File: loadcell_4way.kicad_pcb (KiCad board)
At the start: 2 copper layers, 60 x 40 mm, 76 parts, among them J1 USB_B_Micro, J2 Battery, J3 OLDED_Screen, J4 Load Cell, Q1 FDS6892A, Q2 BSS138, Q3 SM2331PSA P-MOSFET, Q4 S8550, Q5 BSS138, SW1 SW_Push, SW2 SW_Push, SW3 SW_Push, U1 FS312F-G, U2 MT3608, U3 TP4056, U4 CH330N, U5 LM1117-3.3, U7 HX711

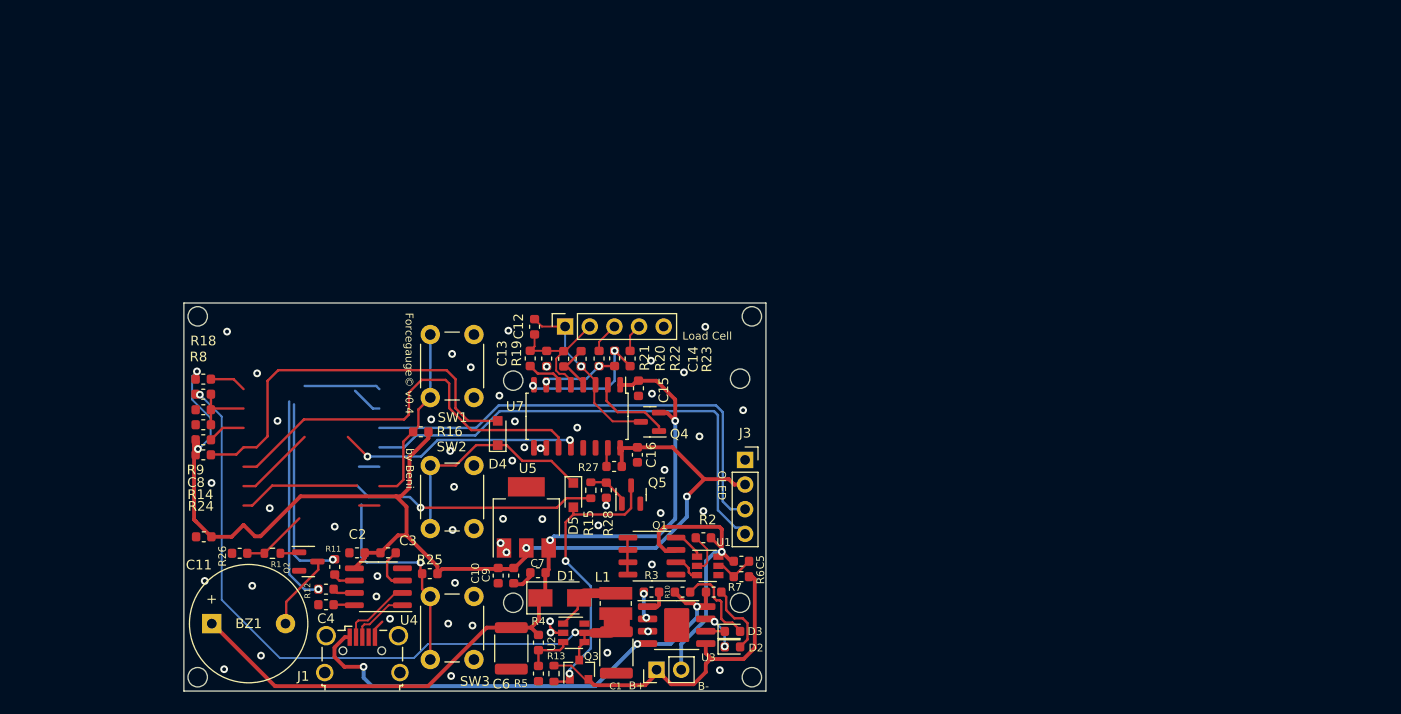
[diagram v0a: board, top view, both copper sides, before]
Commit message: wip
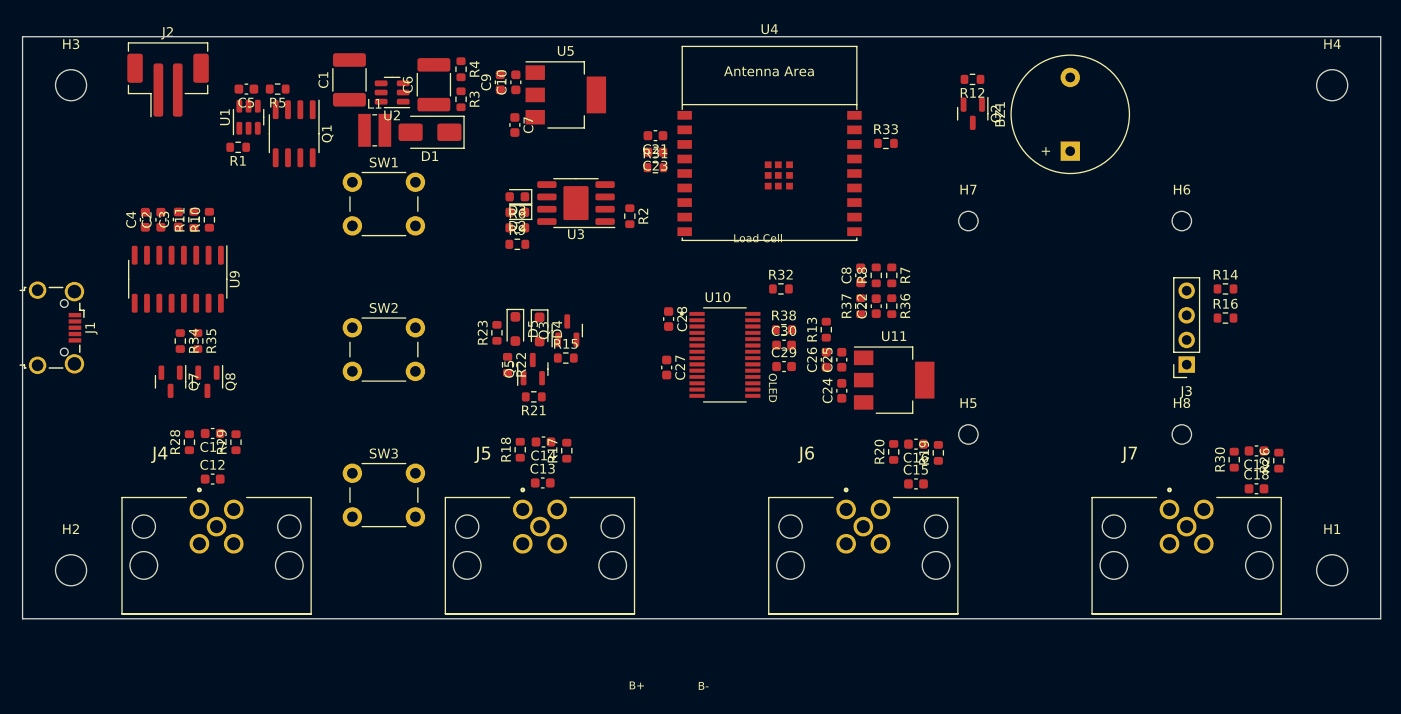
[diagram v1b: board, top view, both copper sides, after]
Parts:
- removed C11: 100nF, Capacitor_SMD:C_0603_1608Metric
- removed Q4: S8550, Package_TO_SOT_SMD:SOT-23
- removed R24: 100k, Resistor_SMD:R_0603_1608Metric
- removed R25: 10k, Resistor_SMD:R_0603_1608Metric
- removed R27: 0R, Resistor_SMD:R_0603_1608Metric
- removed U7: HX711, Package_SO:SOP-16_4.55x10.3mm_P1.27mm
- added C17: 100nF, Capacitor_SMD:C_0603_1608Metric, F.Cu at (119.6, 80.9)
- added C18: 100nF, Capacitor_SMD:C_0603_1608Metric, F.Cu at (227.2, 86.6)
- added C19: 100nF, Capacitor_SMD:C_0603_1608Metric, F.Cu at (227.2, 82.7)
- added C21: 100nF, Capacitor_SMD:C_0603_1608Metric, F.Cu at (165.2, 50.2)
- added C22: 100nF, Capacitor_SMD:C_0603_1608Metric, F.Cu at (188.0, 67.8)
- added C23: 10uF, Capacitor_SMD:C_0603_1608Metric, F.Cu at (165.2, 51.9)
- added C24: 10uF, Capacitor_SMD:C_0603_1608Metric, F.Cu at (184.4, 76.5)
- added C25: 10uF, Capacitor_SMD:C_0603_1608Metric, F.Cu at (184.4, 73.3)
- added C26: 100nF, Capacitor_SMD:C_0603_1608Metric, F.Cu at (182.8, 73.3)
- added C27: 100nF, Capacitor_SMD:C_0603_1608Metric, F.Cu at (166.4, 74.1)
- added C28: 100nF, Capacitor_SMD:C_0603_1608Metric, F.Cu at (166.6, 69.1)
- added C29: 100nF, Capacitor_SMD:C_0603_1608Metric, F.Cu at (178.5, 74.0)
- added C30: 100nF, Capacitor_SMD:C_0603_1608Metric, F.Cu at (178.5, 71.8)
- added J5: T4145015051-001, Loadcell:TE_T4145015051-001, F.Cu at (153.3, 90.5)
- added J6: T4145015051-001, Loadcell:TE_T4145015051-001, F.Cu at (186.7, 90.5)
- added J7: T4145015051-001, Loadcell:TE_T4145015051-001, F.Cu at (220.0, 90.5)
- added Q7: BSS138, Package_TO_SOT_SMD:SOT-23, F.Cu at (115.3, 75.6)
- added Q8: BSS138, Package_TO_SOT_SMD:SOT-23, F.Cu at (119.1, 75.6)
- added R17: 1k, Resistor_SMD:R_0603_1608Metric, F.Cu at (156.1, 82.7)
- added R29: 1k, Resistor_SMD:R_0603_1608Metric, F.Cu at (122.0, 81.8)
- added R30: 1k, Resistor_SMD:R_0603_1608Metric, F.Cu at (224.9, 83.6)
- added R31: 10k, Resistor_SMD:R_0603_1608Metric, F.Cu at (165.2, 53.5)
- added R32: 10k, Resistor_SMD:R_0603_1608Metric, F.Cu at (178.2, 66.0)
- added R33: 10k, Resistor_SMD:R_0603_1608Metric, F.Cu at (189.0, 51.0)
- added R34: 10k, Resistor_SMD:R_0603_1608Metric, F.Cu at (116.3, 71.4)
- added R35: 10k, Resistor_SMD:R_0603_1608Metric, F.Cu at (118.1, 71.4)
- added R36: 390k, Resistor_SMD:R_0603_1608Metric, F.Cu at (189.6, 67.8)
- added R37: 100k, Resistor_SMD:R_0603_1608Metric, F.Cu at (186.4, 67.8)
- added R38: 10k, Resistor_SMD:R_0603_1608Metric, F.Cu at (178.5, 70.2)
- added U10: ADS1234IPW, Loadcell:SOP65P640X120-28N, F.Cu at (172.4, 72.8)
- added U11: LM1117-3.3, Package_TO_SOT_SMD:SOT-223, F.Cu at (189.8, 75.4)
- added U9: CH340C, Package_SO:SOIC-16_3.9x9.9mm_P1.27mm, F.Cu at (116.0, 65.0)
- C12, C15: value 10uF -> 100nF
- H1, H2, H3, H4: value MountingHole -> PCB Mounting hole; footprint forcegauge:MountingHole_2mm_OLED -> MountingHole:MountingHole_3.2mm_M3
- H5, H6, H7, H8: value PCB Mounting hole -> MountingHole; footprint forcegauge:MountingHole_2mm_OLED -> Loadcell:MountingHole_2mm_OLED
- J2: footprint Connector_PinHeader_2.54mm:PinHeader_1x02_P2.54mm_Vertical -> Connector_JST:JST_PH_B2B-PH-SM4-TB_1x02-1MP_P2.00mm_Vertical
- J4: value Load Cell -> T4145015051-001; footprint Connector_PinSocket_2.54mm:PinSocket_1x05_P2.54mm_Vertical -> Loadcell:TE_T4145015051-001
- R1: value 100 -> 2k
- R10: value 1k -> 470R
- R12: value 470R -> 100
- R13: value 100k -> 0R
- R14, R16: value 10k -> 4k7
- R15: value 100 -> 100k
- R18, R26, R28: value 10k -> 1k
- R19: value 0R -> 1k
- R20: value 20k -> 1k
- R21: value 8k2 -> 10k
- R22, R5: value 1k -> 100
- R23: value 1k -> 100k
- R3: value 2k -> 7.5k
- R4: value 7.5k -> 1k
- R6: value 100 -> 1k
- R7: value 1k -> 390k
- R8: value 390k -> 100k
- R9: value 100k -> 1k
- U3: footprint forcegauge:SOP8-PP -> Loadcell:SOP8-PP
- U4: value CH330N -> ESP32-C3-WROOM-02; footprint Package_SO:SOIC-8_3.9x4.9mm_P1.27mm -> Loadcell:ESP32-C3-WROOM-02
- moved R26 107.5 mm to (229.5, 83.7), turned to 90 degrees
- moved R14 106.5 mm to (224.0, 66.0)
- moved BZ1 101.0 mm to (208.0, 51.8), turned to 90 degrees
- moved R12 84.9 mm to (197.9, 44.4)
- moved R16 83.8 mm to (224.0, 69.0), turned to 0 degrees
- moved H5 83.3 mm to (197.5, 81.0)
- moved Q2 82.6 mm to (197.9, 47.9), turned to -90 degrees
- moved H4 81.1 mm to (235.0, 45.0), turned to 0 degrees
- moved H7 80.1 mm to (197.5, 59.0)
- moved J2 78.5 mm to (115.0, 45.0), turned to 0 degrees
- moved C5 70.5 mm to (123.1, 45.4)
- moved R8 70.4 mm to (188.0, 64.6), turned to 90 degrees
- moved H3 70.2 mm to (105.0, 45.0), turned to 0 degrees
- moved C8 69.5 mm to (186.4, 64.6), turned to 90 degrees
- moved U1 66.2 mm to (123.3, 48.3), turned to 90 degrees
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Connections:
- BZ1 pad 2: (no net) -> Net-(BZ1-+)
- C12 pad 1: E- -> +3.3VA
- C12 pad 2: E+ -> Net-(C12-Pad2)
- C13 pad 1: (no net) -> +3.3VA
- C13 pad 2: E- -> Net-(C13-Pad2)
- C14 pad 1: (no net) -> A2+
- C14 pad 2: (no net) -> A2-
- C15 pad 1: GND -> +3.3VA
- C15 pad 2: +5V -> Net-(C15-Pad2)
- C16 pad 1: +3V3 -> A3+
- C16 pad 2: GND -> A3-
- C4 pad 1: (no net) -> +3V3
- C5 pad 1: (no net) -> Net-(U1-VCC)
- C8 pad 1: V_BAT -> VBAT_FB
- D1 pad 2: (no net) -> Net-(D1-A)
- D2 pad 1: (no net) -> Net-(D2-K)
- D2 pad 2: (no net) -> Net-(D2-A)
- D3 pad 1: (no net) -> Net-(D3-K)
- D3 pad 2: (no net) -> Net-(D3-A)
- D4 pad 1: (no net) -> Net-(D4-K)
- D4 pad 2: BTN_2 -> Net-(D4-A)
- D5 pad 1: (no net) -> Net-(D4-K)
- D5 pad 2: (no net) -> BTN_2
- J1 pad 4: (no net) -> unconnected-(J1-ID-Pad4)
- J3 pad 3: SCL -> ESP32_IO9
- J4 pad 1: E+ -> +3.3VA
- J4 pad 2: E- -> Net-(C12-Pad2)
- J4 pad 3: A- -> Net-(J4-Pad3)
- J4 pad 4: A+ -> Net-(J4-Pad4)
- L1 pad 2: (no net) -> Net-(D1-A)
- Q1 pad 2: (no net) -> Net-(Q1A-G1)
- Q1 pad 4: (no net) -> Net-(Q1B-G2)
- Q1 pad 5: (no net) -> Net-(Q1A-D1-Pad7)
- Q1 pad 6: (no net) -> Net-(Q1A-D1-Pad7)
- Q1 pad 7: (no net) -> Net-(Q1A-D1-Pad7)
- Q1 pad 8: (no net) -> Net-(Q1A-D1-Pad7)
- Q2 pad 1: (no net) -> Net-(Q2-G)
- Q2 pad 3: (no net) -> Net-(BZ1-+)
- Q3 pad 1: (no net) -> Net-(D4-A)
- Q5 pad 1: (no net) -> Net-(Q5-G)
- Q5 pad 3: (no net) -> Net-(D4-A)
- R1 pad 1: (no net) -> Net-(U1-CS)
- R1 pad 2: BUZZER -> BAT-
- R10 pad 1: (no net) -> Net-(U9-TXD)
- R10 pad 2: VBUS -> RXD
- R11 pad 1: (no net) -> Net-(U9-RXD)
- R11 pad 2: RXD -> TXD
- R12 pad 1: (no net) -> Net-(Q2-G)
- R12 pad 2: TXD -> BUZZER
- R13 pad 1: (no net) -> GNDA
- R13 pad 2: BAT+ -> GND
- R14 pad 1: +3V3 -> SDA
- R14 pad 2: (no net) -> +3V3
- R15 pad 1: PWR_EN -> Net-(D4-A)
- R15 pad 2: (no net) -> BAT+
- R16 pad 1: +3V3 -> ESP32_IO9
- R16 pad 2: BTN_1 -> +3V3
- R18 pad 1: +3V3 -> Net-(J5-Pad4)
- R18 pad 2: (no net) -> A2-
- R19 pad 1: E- -> Net-(J6-Pad3)
- R19 pad 2: GND -> A3+
- R2 pad 1: (no net) -> Net-(U3-PROG)
- R2 pad 2: BAT- -> GND
- R20 pad 1: E+ -> Net-(J6-Pad4)
- R20 pad 2: (no net) -> A3-
- R21 pad 1: (no net) -> GND
- R21 pad 2: E- -> Net-(Q5-G)
- R22 pad 1: A- -> PWR_EN
- R22 pad 2: (no net) -> Net-(Q5-G)
- R23 pad 1: A+ -> BTN_2
- R23 pad 2: (no net) -> +3V3
- R26 pad 1: GND -> Net-(J7-Pad3)
- R26 pad 2: BUZZER -> A4+
- R28 pad 1: GND -> Net-(J4-Pad4)
- R28 pad 2: (no net) -> A1-
- R3 pad 1: (no net) -> Net-(U2-FB)
- R3 pad 2: GND -> +5V
- R4 pad 1: (no net) -> GND
- R4 pad 2: +5V -> Net-(U2-FB)
- R5 pad 1: GND -> BAT+
- R5 pad 2: (no net) -> Net-(U1-VCC)
- R6 pad 1: BAT+ -> Net-(D2-A)
- R6 pad 2: (no net) -> VBUS
- R7 pad 1: (no net) -> VCC
- R7 pad 2: VBUS -> VBAT_FB
- R8 pad 1: VCC -> VBAT_FB
- R8 pad 2: V_BAT -> GND
- R9 pad 1: V_BAT -> Net-(D3-A)
- R9 pad 2: GND -> VBUS
- SW2 pad 1: (no net) -> BTN_3
- SW3 pad 1: BTN_3 -> Net-(D4-K)
- U1 pad 1: (no net) -> Net-(Q1B-G2)
- U1 pad 2: (no net) -> Net-(U1-CS)
- U1 pad 3: (no net) -> Net-(Q1A-G1)
- U1 pad 4: (no net) -> unconnected-(U1-TD-Pad4)
- U1 pad 5: (no net) -> Net-(U1-VCC)
- U2 pad 1: (no net) -> Net-(D1-A)
- U2 pad 3: (no net) -> Net-(U2-FB)
- U2 pad 6: (no net) -> unconnected-(U2-NC-Pad6)
- U3 pad 2: (no net) -> Net-(U3-PROG)
- U3 pad 6: (no net) -> Net-(D3-K)
- U3 pad 7: (no net) -> Net-(D2-K)
- U4 pad 1: D+ -> +3V3
- U4 pad 2: D- -> ESP32_EN
- U4 pad 3: GND -> MUX0
- U4 pad 4: (no net) -> MUX1
- U4 pad 5: +3V3 -> CLK
- U4 pad 6: (no net) -> DOUT
- U4 pad 7: (no net) -> SDA
- U4 pad 8: (no net) -> ESP32_IO9
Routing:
- net (no net): track 182.0 -> 0.00 mm, vias 10 -> 0
- net +3V3: track 121.1 -> 0.00 mm, vias 4 -> 0
- net +5V: track 85.7 -> 0.00 mm, vias 2 -> 0
- net VCC: track 76.5 -> 0.00 mm, vias 2 -> 0
- net VBUS: track 52.7 -> 0.00 mm, vias 3 -> 0
- net SDA: track 49.9 -> 0.00 mm
- net SCL: track 48.5 -> 0.00 mm
- net CLK: track 42.5 -> 0.00 mm
- net BTN_2: track 40.5 -> 0.00 mm
- net PWR_EN: track 38.0 -> 0.00 mm, vias 1 -> 0
- net BAT+: track 34.8 -> 0.00 mm
- net DOUT: track 33.7 -> 0.00 mm, vias 2 -> 0
- net BAT-: track 30.9 -> 0.00 mm, vias 1 -> 0
- net TXD: track 29.3 -> 0.00 mm, vias 1 -> 0
- net BTN_3: track 24.3 -> 0.00 mm, vias 1 -> 0
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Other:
- board size 60 x 40 mm -> 140 x 60 mm
- board text removed: "Forcegauge© v0.4"
- board text removed: "by Beni"
